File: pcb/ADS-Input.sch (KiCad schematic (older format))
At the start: 13 parts, among them J10 Conn_01x02_Male, J13 Conn_01x04_Male, U7 ADS1115IDGS, U8 PCA9306DCTR

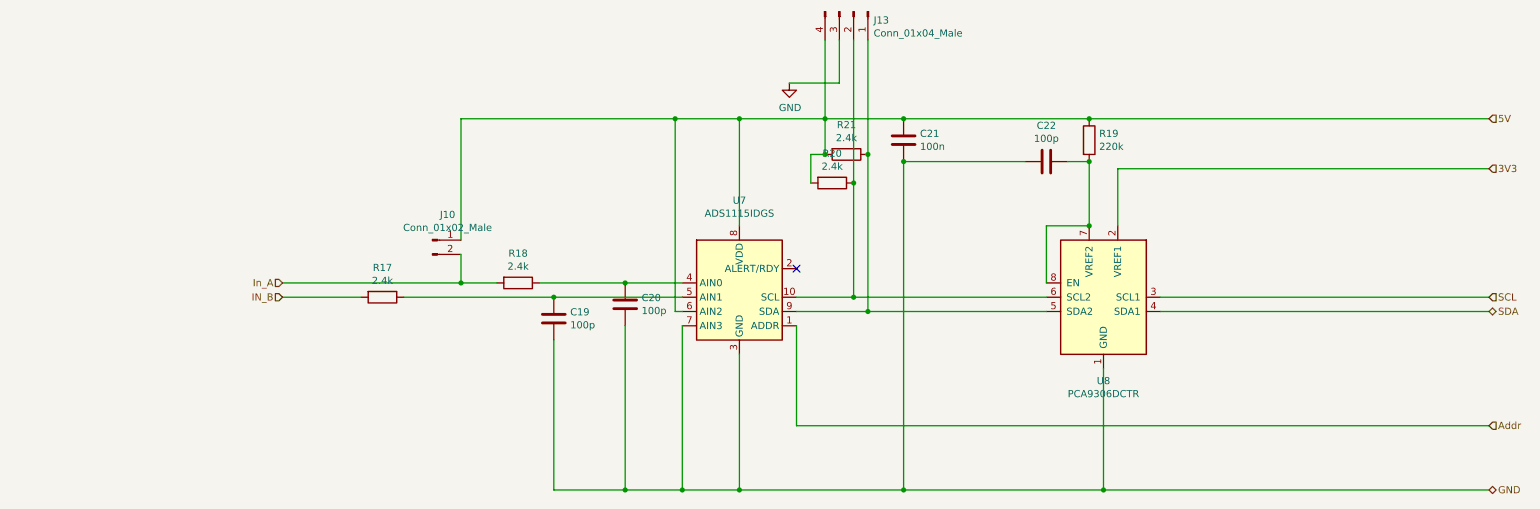
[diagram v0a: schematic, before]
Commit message: first version of the new feature set
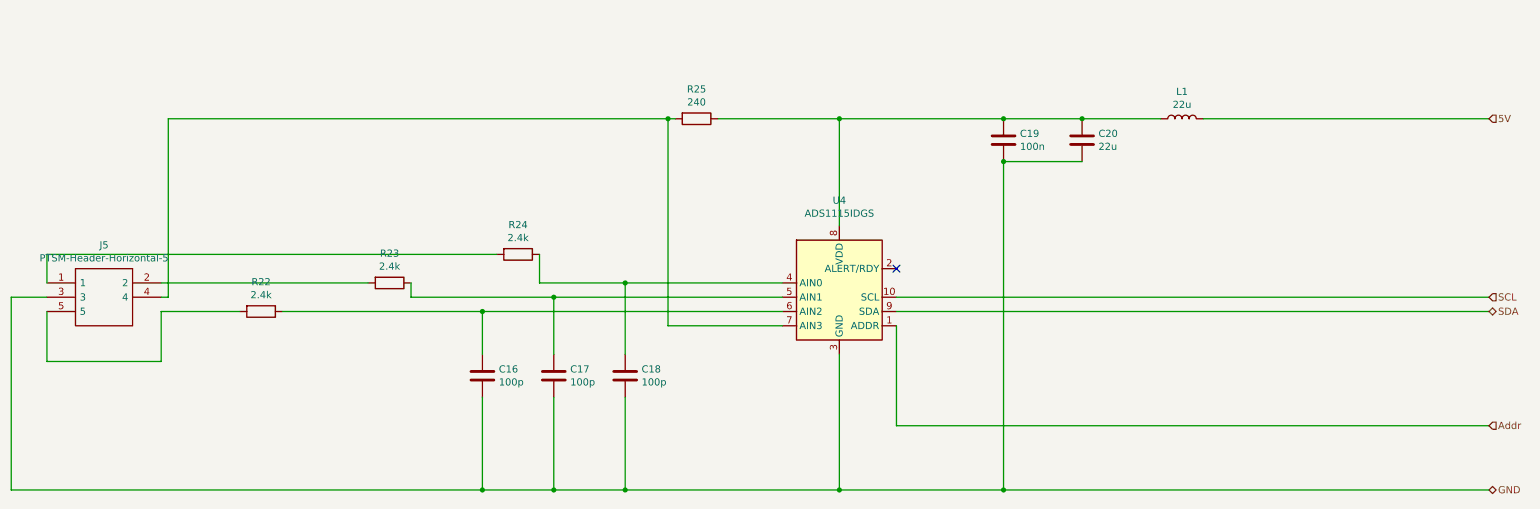
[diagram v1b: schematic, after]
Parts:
- removed C22: 100p, Capacitor_SMD:C_0805_2012Metric_Pad1.15x1.40mm_HandSolder, symbol Device:C
- removed J10: Conn_01x02_Male, Connector_PinHeader_2.54mm:PinHeader_1x02_P2.54mm_Vertical, symbol Connector:Conn_01x02_Male
- removed J13: Conn_01x04_Male, Connector_PinHeader_2.54mm:PinHeader_1x04_P2.54mm_Vertical, symbol Connector:Conn_01x04_Male
- removed R19: 220k, Resistor_SMD:R_0805_2012Metric_Pad1.15x1.40mm_HandSolder, symbol Device:R
- removed R20, R21: 2.4k, Resistor_SMD:R_0805_2012Metric_Pad1.15x1.40mm_HandSolder, symbol Device:R
- removed U8: PCA9306DCTR, Package_SO:SSOP-8_2.95x2.8mm_P0.65mm, symbol Interface:PCA9306
- added C16: 100p, Capacitor_SMD:C_0805_2012Metric, symbol Device:C
- added C20: 22u, Capacitor_SMD:C_0805_2012Metric, symbol Device:C
- added J5: PTSM-Header-Horizontal-5, Connector_own:1814870, symbol Connector_own:PTSM-Header-Horizontal-5
- added L1: 22u, Inductor_SMD:L_0805_2012Metric, symbol Device:L
- added R22: 2.4k, Resistor_SMD:R_0805_2012Metric, symbol Device:R
- added R25: 240, Resistor_SMD:R_0805_2012Metric, symbol Device:R
- C17: renamed from C19; footprint Capacitor_SMD:C_0805_2012Metric_Pad1.15x1.40mm_HandSolder -> Capacitor_SMD:C_0805_2012Metric
- C18: renamed from C20; footprint Capacitor_SMD:C_0805_2012Metric_Pad1.15x1.40mm_HandSolder -> Capacitor_SMD:C_0805_2012Metric
- C19: renamed from C21; footprint Capacitor_SMD:C_0805_2012Metric_Pad1.15x1.40mm_HandSolder -> Capacitor_SMD:C_0805_2012Metric
- R23: renamed from R17; footprint Resistor_SMD:R_0805_2012Metric_Pad1.15x1.40mm_HandSolder -> Resistor_SMD:R_0805_2012Metric
- R24: renamed from R18; footprint Resistor_SMD:R_0805_2012Metric_Pad1.15x1.40mm_HandSolder -> Resistor_SMD:R_0805_2012Metric
- renumbered U7 to U4
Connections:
- net 5V: now also L1.2; no longer C19.1, U4.6 (AIN2), U4.8 (VDD)
- net GND: now also C16.2, C20.2, J5.3; no longer U4.7 (AIN3)
- net SCL: now also U4.10 (SCL)
- net SDA: now also U4.9 (SDA)
- net IN_B: no longer names the net of R23.2
- net IN_B: now also J5.2
- net In_A: no longer names the net of R24.2
- net In_A: now also J5.1
- new net: C19.1, C20.1, L1.1, R25.1, U4.8 (VDD)
- new net: C16.1, R22.1, U4.6 (AIN2)
- new net: J5.4, R25.2, U4.7 (AIN3)
- new net: J5.5, R22.2
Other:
- moved on the sheet: C17, C18, C19, R23, R24, U4
